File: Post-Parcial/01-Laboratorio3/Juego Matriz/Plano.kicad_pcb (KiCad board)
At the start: 2 copper layers, 33 parts, among them J1 Conn_01x12, J2 Conn_01x12, J3 Conn_01x19, J4 Conn_01x19, Q1 2N3904, Q2 2N3904, Q3 2N3904, Q4 2N3904, Q5 2N3904, Q6 2N3904, Q7 2N3904, Q8 2N3904, Q9 2N3904, SW1 SW_Push, SW2 SW_Push, SW3 SW_DPST_x2

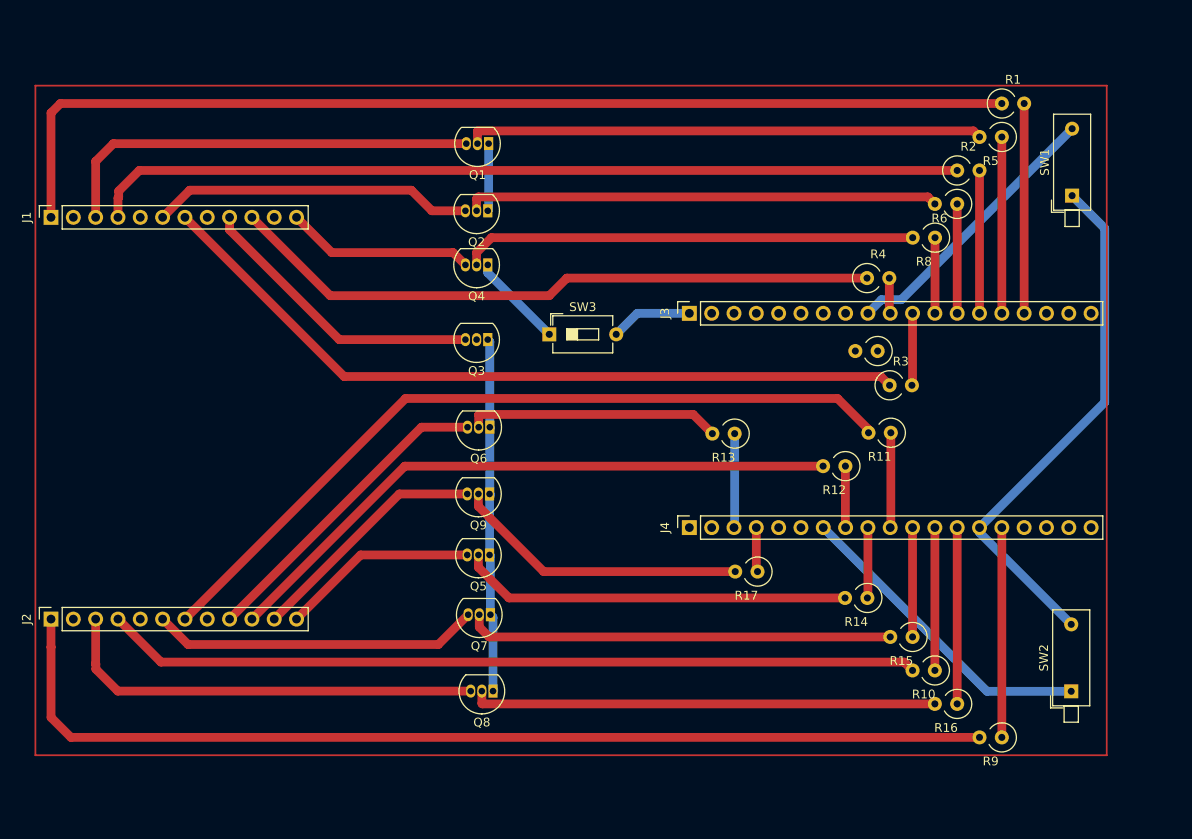
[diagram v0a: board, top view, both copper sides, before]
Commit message: PCB Juego Finalizado
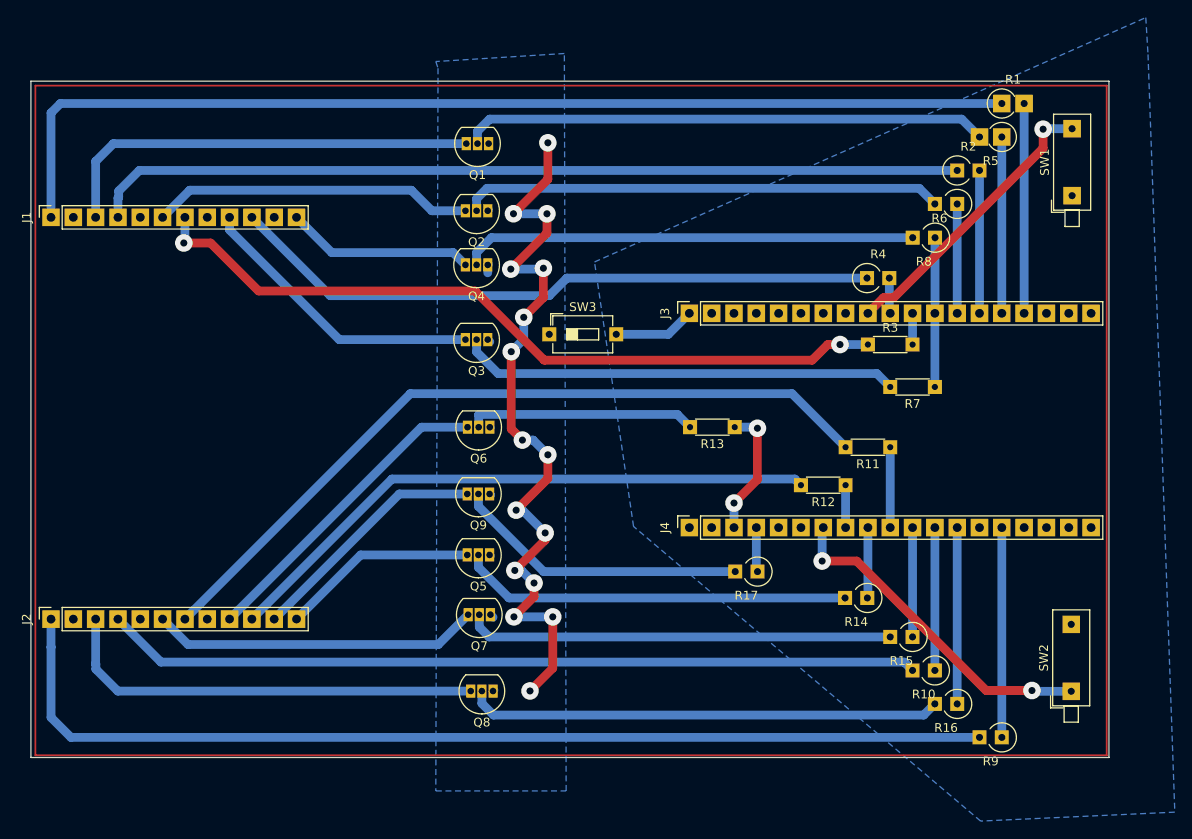
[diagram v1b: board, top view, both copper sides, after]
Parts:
- R11, R12, R13, R3, R7: footprint Resistor_THT:R_Axial_DIN0309_L9.0mm_D3.2mm_P2.54mm_Vertical -> Resistor_THT:R_Axial_DIN0204_L3.6mm_D1.6mm_P5.08mm_Horizontal
- moved R7 7.69 mm to (198.9, 97.8)
- moved R3 5.25 mm to (191.3, 93.0)
- moved R12 2.17 mm to (188.7, 109.0)
- moved R11 1.65 mm to (193.8, 104.6)
- moved R13 0.74 mm to (176.1, 102.4)
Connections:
- Q1 pad 1: GND -> GND_BJT
- Q2 pad 1: GND -> GND_BJT
- Q3 pad 1: GND -> GND_BJT
- Q4 pad 1: Net-(Q4-E) -> GND_BJT
- Q5 pad 1: GND -> GND_BJT
- Q6 pad 1: GND -> GND_BJT
- Q7 pad 1: GND -> GND_BJT
- Q8 pad 1: GND -> GND_BJT
- Q9 pad 1: GND -> GND_BJT
- SW3 pad 1: Net-(Q4-E) -> GND_BJT
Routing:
- net GND: track 118.2 -> 9.31 mm
- net GND_BJT: track 0.00 -> 92.9 mm, vias 0 -> 16
- net Net-(Q3-B): track 0.00 -> 50.1 mm
- net Net-(Q4-E): track 10.8 -> 0.00 mm
- net GPIO16: track 8.62 -> 17.0 mm
- net Net-(J3-Pin_11): track 8.22 -> 3.56 mm
- net GPI36: track 10.7 -> 15.2 mm, vias 0 -> 2
- net Net-(Q6-B): track 28.9 -> 26.1 mm
- net GPIO33: track 72.2 -> 69.4 mm
- net GPIO32: track 35.9 -> 38.3 mm, vias 0 -> 2
- net Net-(J4-Pin_8): track 7.00 -> 4.83 mm
- net GPIO26: track 90.0 -> 88.3 mm
- net Net-(J4-Pin_10): track 10.8 -> 9.14 mm
- net GPIO18: track 31.9 -> 33.2 mm, vias 0 -> 1
- net Net-(Q1-B): track 58.8 -> 60.0 mm
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- added copper zone on B.Cu, net GND
- added copper zone on B.Cu, net GND_BJT
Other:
- board outline added: 122.7 x 77 mm
